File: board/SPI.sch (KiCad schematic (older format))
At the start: 28 parts, among them P3 CONN_7X2, U11 MICRO_SD, U17 FXO-HC536R, U3 W25Q128FVEIG

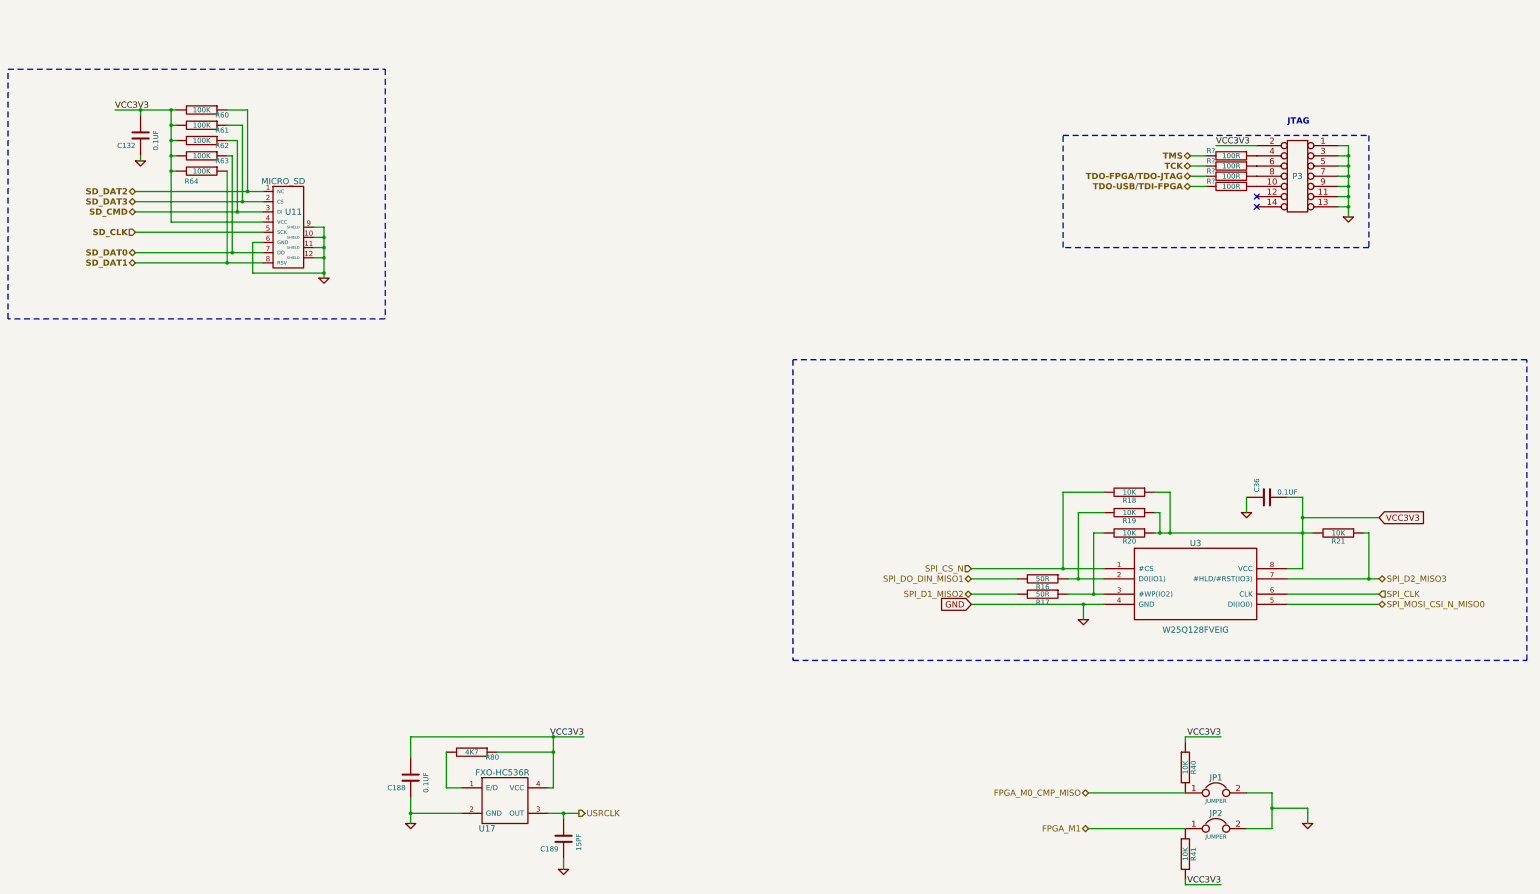
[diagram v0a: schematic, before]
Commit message: Issue #1458 - USB2.0
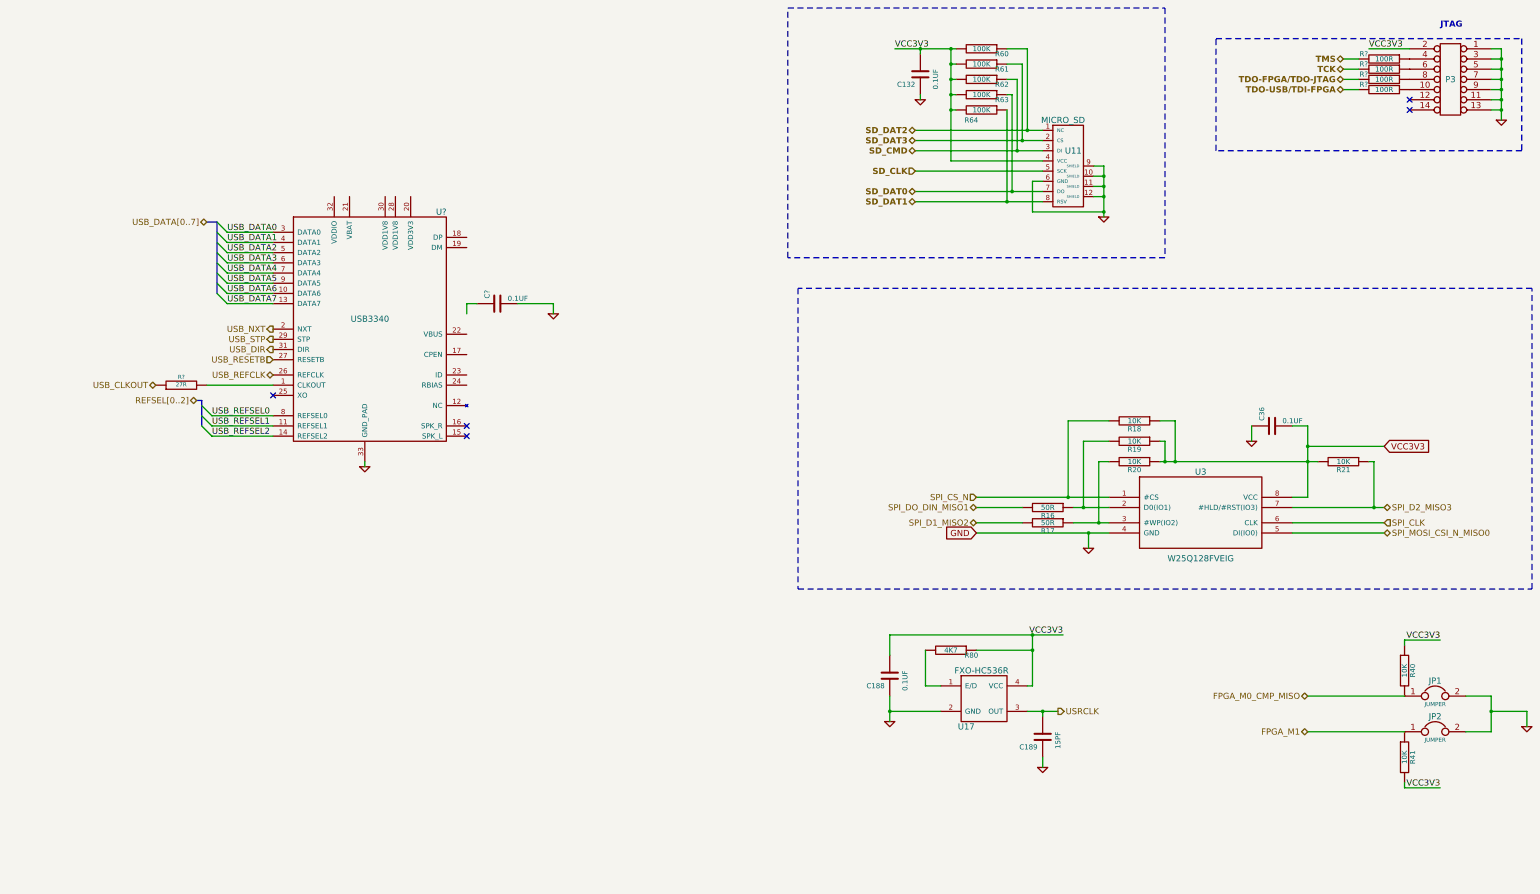
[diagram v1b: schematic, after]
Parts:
- added C?: 0.1UF, symbol C
- added R?: 27R, ~, symbol R
- added U?: USB3340, symbol USB3340
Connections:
- net GND: now also C?.2, U?.33 (GND_PAD)
- new net: R?.2, U?.1 (CLKOUT)
- new net USB_CLKOUT: R?.1
- new net USB_DATA0: U?.3 (DATA0)
- new net USB_DATA1: U?.4 (DATA1)
- new net USB_DATA2: U?.5 (DATA2)
- new net USB_DATA3: U?.6 (DATA3)
- new net USB_DATA4: U?.7 (DATA4)
- new net USB_DATA5: U?.9 (DATA5)
- new net USB_DATA6: U?.10 (DATA6)
- new net USB_DATA7: U?.13 (DATA7)
- new net USB_DIR: U?.31 (DIR)
- new net USB_NXT: U?.2 (NXT)
- new net USB_REFCLK: U?.26 (REFCLK)
- new net USB_REFSEL0: U?.8 (REFSEL0)
- new net USB_REFSEL1: U?.11 (REFSEL1)
- new net USB_REFSEL2: U?.14 (REFSEL2)
- new net USB_RESETB: U?.27 (RESETB)
- new net USB_STP: U?.29 (STP)
- no-connect marks 2 -> 5
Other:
- moved on the sheet: C132, C188, C189, C36, JP1, JP2, P3, R16, R17, R18, R19, R20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
